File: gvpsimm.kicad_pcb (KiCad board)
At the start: 4 copper layers, 97.8 x 22.2 mm, 18 parts, among them J1 SIMM64_EDGE, U1 HM514400_alt, U2 HM514400_alt, U3 HM514400_alt, U4 HM514400_alt, U5 HM514400_alt, U6 HM514400_alt, U7 HM514400_alt, U8 HM514400_alt

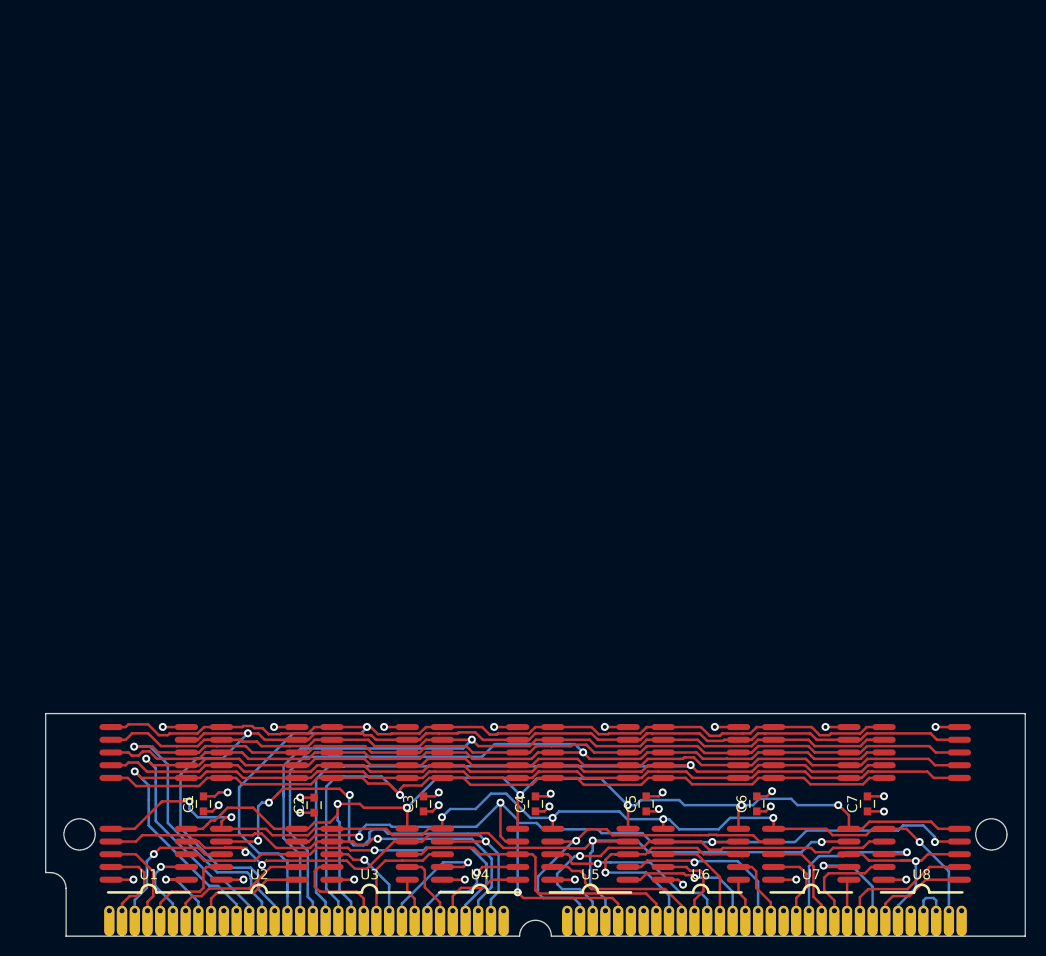
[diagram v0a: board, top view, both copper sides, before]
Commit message: 16MB study
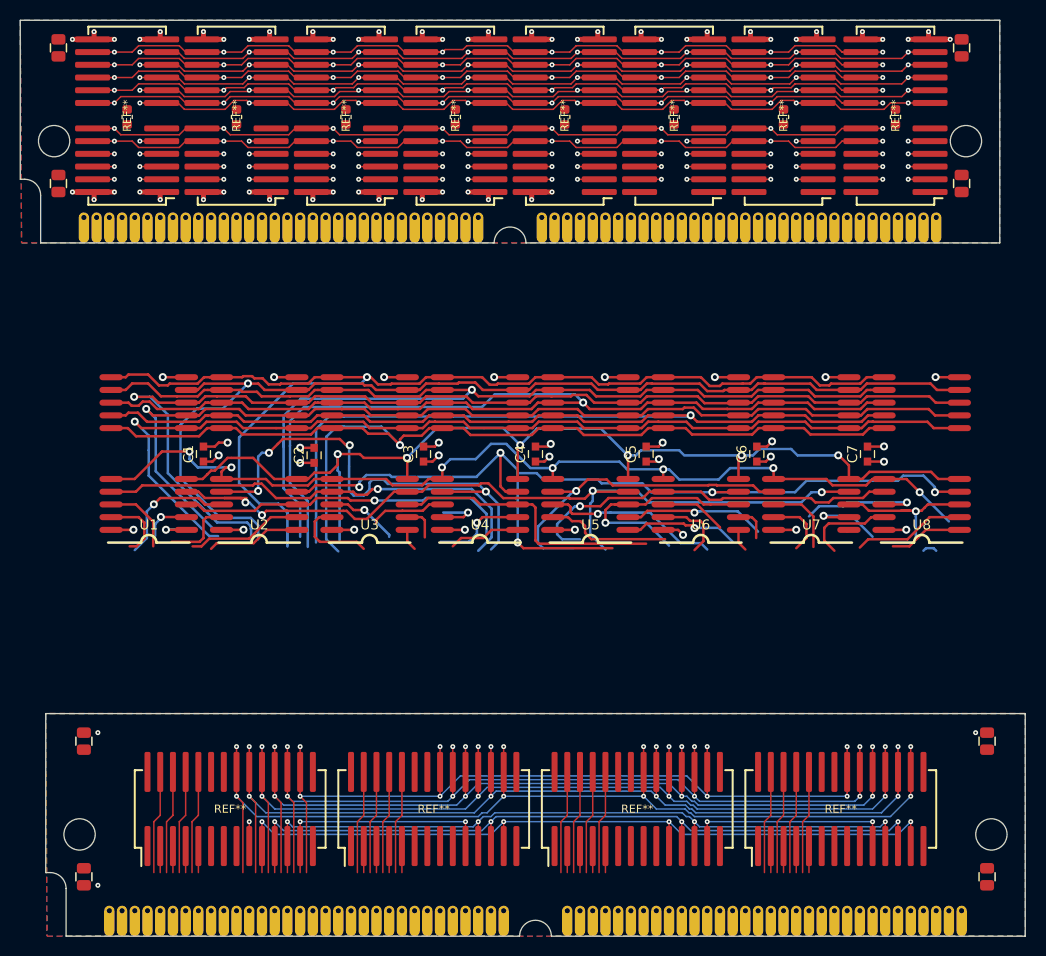
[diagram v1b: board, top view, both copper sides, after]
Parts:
- added H1: MountingHole, Conn:MH_125, F.Cu at (104.3, 9.53)
- added H2: MountingHole, Conn:MH_125, F.Cu at (195.4, 9.53)
- added J1: SIMM64_EDGE, Conn:EDGE_SIMM_64_127, F.Cu at (149.9, 19.7)
- added REF**: SOJ-24-26-300mil-Skinny, stdpads:SOJ-24-26-300mil-Skinny, F.Cu at (188.3, 6.99)
- added REF**: C_0603, stdpads:C_0603, F.Cu at (155.3, 7.11)
- added REF**: C_0603, stdpads:C_0603, F.Cu at (144.4, 7.11)
- added REF**: C_0603, stdpads:C_0603, F.Cu at (166.2, 7.11)
- added REF**: C_0805, stdpads:C_0805, F.Cu at (104.8, 0.21)
- added REF**: C_0805, stdpads:C_0805, F.Cu at (104.8, 13.8)
- added REF**: C_0805, stdpads:C_0805, F.Cu at (194.9, 13.8)
- added REF**: C_0805, stdpads:C_0805, F.Cu at (194.9, 0.21)
- added REF**: C_0603, stdpads:C_0603, F.Cu at (111.6, 7.11)
- added REF**: C_0603, stdpads:C_0603, F.Cu at (122.6, 7.11)
- added REF**: C_0603, stdpads:C_0603, F.Cu at (188.3, 7.11)
- added REF**: SOJ-24-26-300mil-Skinny, stdpads:SOJ-24-26-300mil-Skinny, F.Cu at (177.2, 6.99)
- added REF**: C_0603, stdpads:C_0603, F.Cu at (133.5, 7.11)
- added REF**: SOJ-28-300mil, stdpads:SOJ-28-300mil, F.Cu at (182.9, 76.2)
- added REF**: SOJ-28-300mil, stdpads:SOJ-28-300mil, F.Cu at (162.6, 76.2)
- added REF**: SOJ-28-300mil, stdpads:SOJ-28-300mil, F.Cu at (142.2, 76.2)
- added REF**: SOJ-28-300mil, stdpads:SOJ-28-300mil, F.Cu at (121.9, 76.2)
- added REF**: C_0805, stdpads:C_0805, F.Cu at (197.5, 69.4)
- added REF**: C_0805, stdpads:C_0805, F.Cu at (197.5, 83.0)
- added REF**: C_0805, stdpads:C_0805, F.Cu at (107.3, 83.0)
- added REF**: C_0805, stdpads:C_0805, F.Cu at (107.3, 69.4)
- added REF**: SOJ-24-26-300mil-Skinny, stdpads:SOJ-24-26-300mil-Skinny, F.Cu at (155.3, 6.99)
- added REF**: SOJ-24-26-300mil-Skinny, stdpads:SOJ-24-26-300mil-Skinny, F.Cu at (144.4, 6.99)
- added REF**: SOJ-24-26-300mil-Skinny, stdpads:SOJ-24-26-300mil-Skinny, F.Cu at (166.2, 6.99)
- added REF**: SOJ-24-26-300mil-Skinny, stdpads:SOJ-24-26-300mil-Skinny, F.Cu at (133.5, 6.99)
- added REF**: SOJ-24-26-300mil-Skinny, stdpads:SOJ-24-26-300mil-Skinny, F.Cu at (122.6, 6.99)
- added REF**: SOJ-24-26-300mil-Skinny, stdpads:SOJ-24-26-300mil-Skinny, F.Cu at (111.6, 6.99)
- added REF**: C_0603, stdpads:C_0603, F.Cu at (177.2, 7.11)
- moved C2 34.9 mm to (130.3, 40.9)
- moved U1 34.9 mm to (113.8, 40.7)
- moved U2 34.9 mm to (124.8, 40.7)
- moved U3 34.9 mm to (135.8, 40.7)
- moved U4 34.9 mm to (146.9, 40.7)
- moved U5 34.9 mm to (157.9, 40.7)
- moved U6 34.9 mm to (168.9, 40.7)
- moved U7 34.9 mm to (179.9, 40.7)
- moved U8 34.9 mm to (191.0, 40.7)
- moved C1 34.9 mm to (119.3, 40.8)
- moved C3 34.9 mm to (141.2, 40.8)
- moved C4 34.9 mm to (152.4, 40.8)
- moved C5 34.9 mm to (163.4, 40.8)
- moved C6 34.9 mm to (174.5, 40.8)
- moved C7 34.9 mm to (185.5, 40.8)
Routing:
- net (no net): track 0.00 -> 1320.9 mm, vias 0 -> 208
- net /A0: track 104.9 -> 200.1 mm, vias 1 -> 9
- net /A1: track 105.3 -> 196.7 mm, vias 1 -> 9
- net /A3: track 108.8 -> 198.7 mm, vias 1 -> 9
- net /A5: track 117.4 -> 204.9 mm, vias 1 -> 9
- net /A7: track 133.7 -> 218.5 mm, vias 1 -> 9
- net /A9: track 110.3 -> 191.8 mm, vias 6 -> 14
- net /A2: track 110.8 -> 187.7 mm, vias 1 -> 5
- net /A4: track 114.5 -> 189.6 mm, vias 1 -> 5
- net /A6: track 127.9 -> 200.0 mm, vias 1 -> 5
- net /A8: track 104.2 -> 148.7 mm, vias 1 -> 5
- net /DQ18: track 18.8 -> 28.0 mm
- net /DQ12: track 3.40 -> 12.5 mm
- net /DQ8: track 10.0 -> 19.1 mm
- net /DQ2: track 9.07 -> 17.7 mm
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- added copper zone on B.Cu, net (none)
- added copper zone on F.Cu, net (none)
- added copper zone on In1.Cu, net (none)
- added copper zone on In2.Cu, net (none)
- added copper zone on B.Cu, net GND
- added copper zone on F.Cu, net GND
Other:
- board size 97.8 x 22.2 mm -> 100.3 x 91.4 mm
- net class Default: clearance 0.2 -> 0.15; trace_width 0.25 -> 0.15; via_dia 0.8 -> 0.5; via_drill 0.4 -> 0.2
- rule pad_to_mask_clearance: 0.051 -> 0.05
- rule solder_mask_min_width: 0.25 -> 0.1
- rule trace_clearance: 0.2 -> 0.15
- rule trace_min: 0.2 -> 0.15
- rule via_min_drill: 0.3 -> 0.2
- rule via_min_size: 0.4 -> 0.5
